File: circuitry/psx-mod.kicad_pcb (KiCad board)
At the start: 2 copper layers, 30 x 29.5 mm, 111 parts, among them J1 Conn_01x04, J10 USB 2.0 Type-C, J11 Conn_01x04, J12 Conn_01x01, J13 Conn_01x01, J4 Conn_01x02, J5 Conn_01x02, J6 Conn_01x01, J7 Conn_01x01, J8 Conn_01x02, J9 Conn_01x04, U1 ATtiny404-SS, U2 Si5351A-B-GT, U3 USBLC6-2SC6, U4 CH340C, U5 74LVC2G04, U6 74LVC2G04, U7 XC6219B332MR, Y1 27MHz

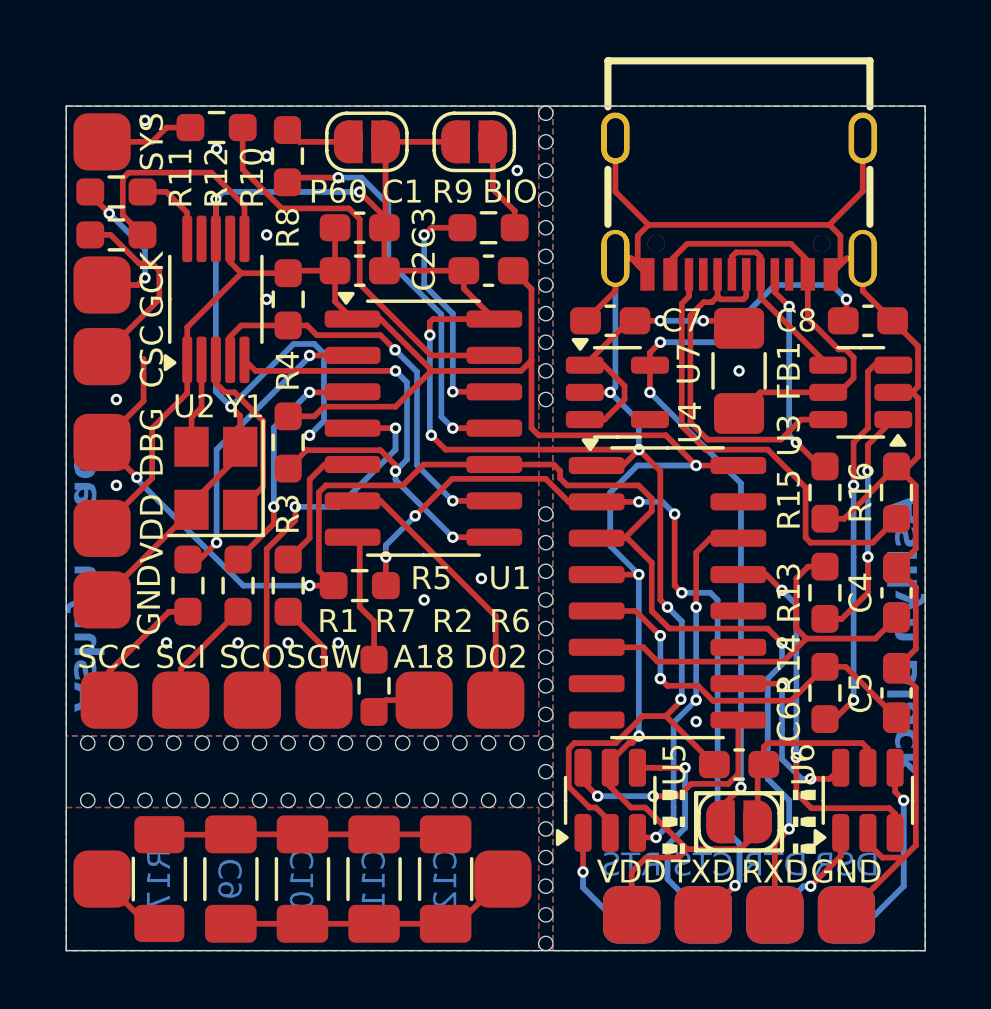
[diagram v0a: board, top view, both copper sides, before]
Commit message: Completed schematic and layout.
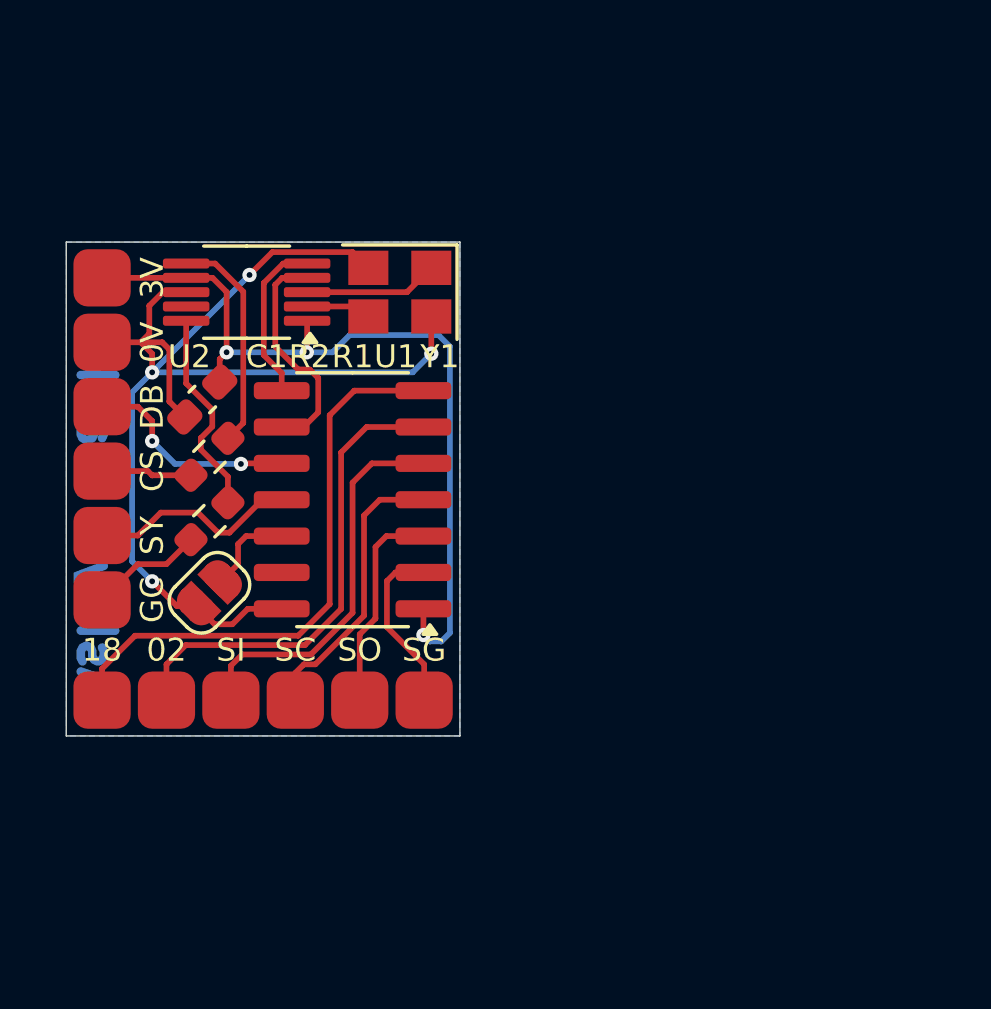
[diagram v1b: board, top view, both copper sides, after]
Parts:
- removed C10, C11, C12, C9: 47µF, Capacitor_SMD:C_1206_3216Metric_Pad1.33x1.80mm_HandSolder
- removed C2, C3, C6, C7, C8: 10µF, Capacitor_SMD:C_0603_1608Metric_Pad1.08x0.95mm_HandSolder
- removed C4, C5: 10pF, Capacitor_SMD:C_0603_1608Metric_Pad1.08x0.95mm_HandSolder
- removed FB1: FerriteBead, Inductor_SMD:L_1206_3216Metric_Pad1.42x1.75mm_HandSolder
- removed J10: USB 2.0 Type-C, PSX_Mod:CONN-SMD_HX-TYPE-C-16PIN
- removed J11, J9: Conn_01x04, PSX_Mod:CONN-SMD_4P
- removed J12, J13, J7: Conn_01x01, PSX_Mod:CONN-SMD_1P
- removed J5, J8: Conn_01x02, PSX_Mod:CONN-SMD_2P
- removed JP2: JMP2O, Jumper:SolderJumper-2_P1.3mm_Open_RoundedPad1.0x1.5mm
- removed JP3: Jumper_2_Open, Jumper:SolderJumper-2_P1.3mm_Open_RoundedPad1.0x1.5mm
- removed the R1 at (139.5, 105.5)
- removed R10, R3, R4, R6, R7, R8, R9: 10kΩ, Resistor_SMD:R_0603_1608Metric_Pad0.98x0.95mm_HandSolder
- removed R13, R14: 10Ω, Resistor_SMD:R_0603_1608Metric_Pad0.98x0.95mm_HandSolder
- removed R15, R16: 5.1kΩ, Resistor_SMD:R_0603_1608Metric_Pad0.98x0.95mm_HandSolder
- removed R17: 75Ω, Resistor_SMD:R_1206_3216Metric_Pad1.30x1.75mm_HandSolder
- removed the R2 at (141.3, 105.5)
- removed R5: 4.7kΩ, Resistor_SMD:R_0603_1608Metric_Pad0.98x0.95mm_HandSolder
- removed REF** (x59): MouseBite, PSX_Mod:MouseBite
- removed U3: USBLC6-2SC6, Package_TO_SOT_SMD:SOT-23-6
- removed U4: CH340C, Package_SO:SOIC-16_3.9x9.9mm_P1.27mm
- removed U5, U6: 74LVC2G04, Package_TO_SOT_SMD:SOT-23-6
- removed U7: XC6219B332MR, Package_TO_SOT_SMD:SOT-23-5
- added J2: Conn_01x04, PSX_Mod:CONN-SMD_4P, F.Cu at (141.0, 109.5)
- added J3: Conn_01x01, PSX_Mod:CONN-SMD_1P, F.Cu at (136.5, 99.2)
- J1: value Conn_01x04 -> Conn_01x02; footprint PSX_Mod:CONN-SMD_4P -> PSX_Mod:CONN-SMD_2P
- J6: value Conn_01x01 -> Conn_01x03; footprint PSX_Mod:CONN-SMD_1P -> PSX_Mod:CONN-SMD_3P
- JP1: value JMP2O -> Jumper_2_Open
- U1: value ATtiny404-SS -> ATtiny414-SS
- moved JP1 16.7 mm to (140.3, 105.8), turned to -135 degrees
- moved J1 15.3 mm to (136.5, 94.8), turned to -90 degrees
- moved J4 12.5 mm to (136.5, 109.5), turned to 0 degrees
- moved R1 12.0 mm to (140.3, 103.2), turned to -135 degrees
- moved Y1 9.14 mm to (146.9, 95.2), turned to 180 degrees
- moved R2 8.40 mm to (140.3, 101.0), turned to -135 degrees
- moved C1 8.14 mm to (140.0, 99.0), turned to -135 degrees
- moved J6 5.50 mm to (136.5, 106.0), turned to 90 degrees
- moved U1 3.52 mm to (145.3, 102.5), turned to 180 degrees
- moved U2 1.10 mm to (141.6, 95.2), turned to 180 degrees
- renumbered R11 to R1, R12 to R2
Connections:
- net Net-(U1-PB0) renamed /scl
- net Net-(U1-PB1) renamed /sda
- J1 pad 1: /scc -> VDD
- J1 pad 2: /sci -> GND
- J4 pad 1: /d02 -> /a18
- J4 pad 2: /a18 -> /d02
- J6 pad 1: /dbg -> /gck
- U1 pad 11: Net-(U1-PA1) -> /sys
- U1 pad 12: Net-(U1-PA2) -> /~{p60}
- U1 pad 13: Net-(U1-PA3) -> unconnected-(U1-PA3-Pad13)
- U1 pad 2: Net-(U1-PA4) -> /scg
- U1 pad 3: Net-(U1-PA5) -> /sco
- U1 pad 4: /sco -> /scc
- U1 pad 5: Net-(U1-PA7) -> /sci
- U1 pad 7: Net-(U1-PB2) -> /a18
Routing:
- net GND: track 142.8 -> 44.1 mm, vias 26 -> 4
- net VDD: track 79.0 -> 29.2 mm
- net /dbg: track 51.8 -> 7.52 mm, vias 4 -> 2
- net /txd: track 29.3 -> 0.00 mm, vias 6 -> 0
- net Net-(JP3-A): track 27.0 -> 0.00 mm, vias 4 -> 0
- net /a18: track 1.92 -> 20.2 mm
- net Net-(J10-CC2): track 16.0 -> 0.00 mm
- net VBUS: track 15.2 -> 0.00 mm
- net Net-(U4-UD-): track 14.7 -> 0.00 mm
- net Net-(U1-PA1): track 14.3 -> 0.00 mm, vias 2 -> 0
- net Net-(U1-PA3): track 14.3 -> 0.00 mm
- net Net-(R14-Pad1): track 13.9 -> 0.00 mm, vias 2 -> 0
- net Net-(U4-UD+): track 13.9 -> 0.00 mm, vias 2 -> 0
- net Net-(U4-~{DTR}): track 13.5 -> 0.00 mm, vias 2 -> 0
- net Net-(J10-D+-PadA6): track 12.9 -> 0.00 mm
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- removed copper zone on B.Cu, net (none)
- removed copper zone on F.Cu, net (none)
- removed copper zone on F.Cu, net GND
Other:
- board size 30 x 29.5 mm -> 13.8 x 17.2 mm
- board text added: "02"
- board text added: "0V"
- board text added: "18"
- board text added: "3V"
- board text added: "CS"
- board text added: "DB"
- board text added: "GC"
- board text added: "SC"
- board text added: "SG"
- board text added: "SI"
- board text added: "SO"
- board text added: "SY"
- board text removed: "!!!"
- board text removed: "A18"
- board text removed: "Ashlyn Black"
- board text removed: "BIO"
- board text removed: "CSC"
- board text removed: "CTS"
- board text removed: "D02"
- board text removed: "DBG"
- board text removed: "DSR"
- board text removed: "DTR"
- board text removed: "GCK"
- board text removed: "GND"
- board text removed: "P60"
- board text removed: "RTS"
- board text removed: "RXD"
- board text removed: "SCC"
- board text removed: "SCI"
- board text removed: "SCO"
- board text removed: "SGW"
- board text removed: "SYS"
- board text removed: "TXD"
- board text removed: "VDD"
